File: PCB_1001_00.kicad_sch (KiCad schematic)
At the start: 10 parts, among them SW1 SW_MEC_5G_edit, SW2 SW_MEC_5G_edit, SW3 SW_MEC_5G_edit

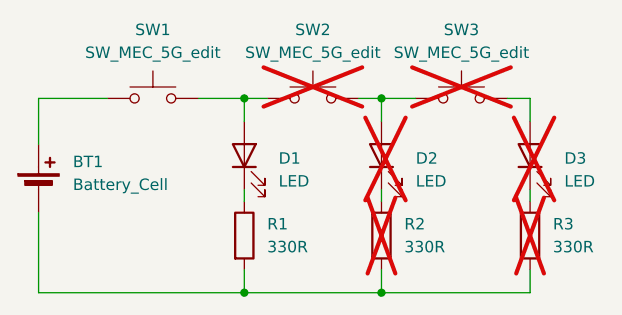
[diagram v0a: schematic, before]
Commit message: PCB_1001_00.kicad_pro fixed
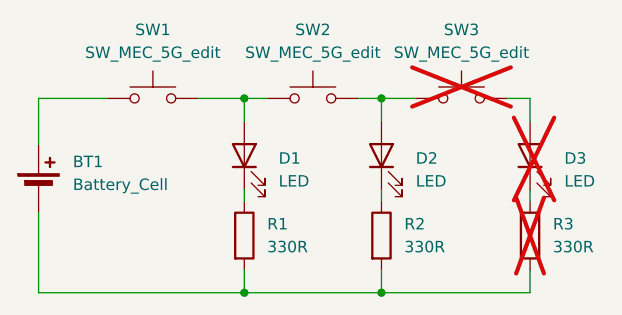
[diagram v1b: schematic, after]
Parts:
- D2, R2, SW2: now fitted
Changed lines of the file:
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@@
 		(in_bom yes)
 		(on_board yes)
-		(dnp yes)
+		(dnp no)
 		(fields_autoplaced yes)
 		(property "Reference" "SW2"
@@
 		(in_bom yes)
 		(on_board yes)
-		(dnp yes)
+		(dnp no)
 		(fields_autoplaced yes)
 		(property "Reference" "R2"
@@
 		(in_bom yes)
 		(on_board yes)
-		(dnp yes)
+		(dnp no)
 		(fields_autoplaced yes)
 		(property "Reference" "D2"

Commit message: VAR_PCA_1002_00 circuit #2 & 3 is DNP
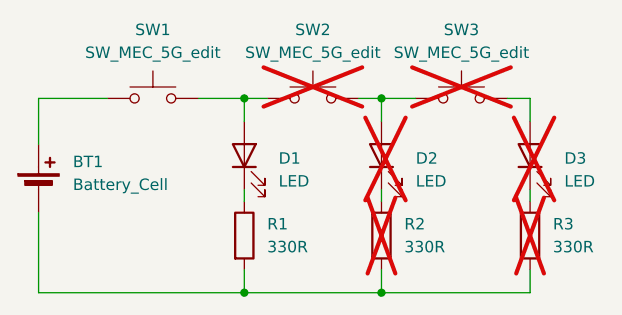
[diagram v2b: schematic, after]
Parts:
- D2, R2, SW2: now not fitted
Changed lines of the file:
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@@
 		(in_bom yes)
 		(on_board yes)
-		(dnp no)
+		(dnp yes)
 		(fields_autoplaced yes)
 		(property "Reference" "SW2"
@@
 		(in_bom yes)
 		(on_board yes)
-		(dnp no)
+		(dnp yes)
 		(fields_autoplaced yes)
 		(property "Reference" "R2"
@@
 		(in_bom yes)
 		(on_board yes)
-		(dnp no)
+		(dnp yes)
 		(fields_autoplaced yes)
 		(property "Reference" "D2"
